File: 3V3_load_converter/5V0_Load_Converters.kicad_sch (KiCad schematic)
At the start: 78 parts, among them J19 N/A, J20 N/A, Q1 SI2302DDS-T1-GE3, Q11 EPC2016C, Q12 EPC2016C, Q2 SI2302DDS-T1-GE3, Q3 EPC2016C, Q4 EPC2016C, U22 INA199C3DCKR, U23 LTC3833EUDC#TRPBF, U26 LTC3833EUDC#TRPBF

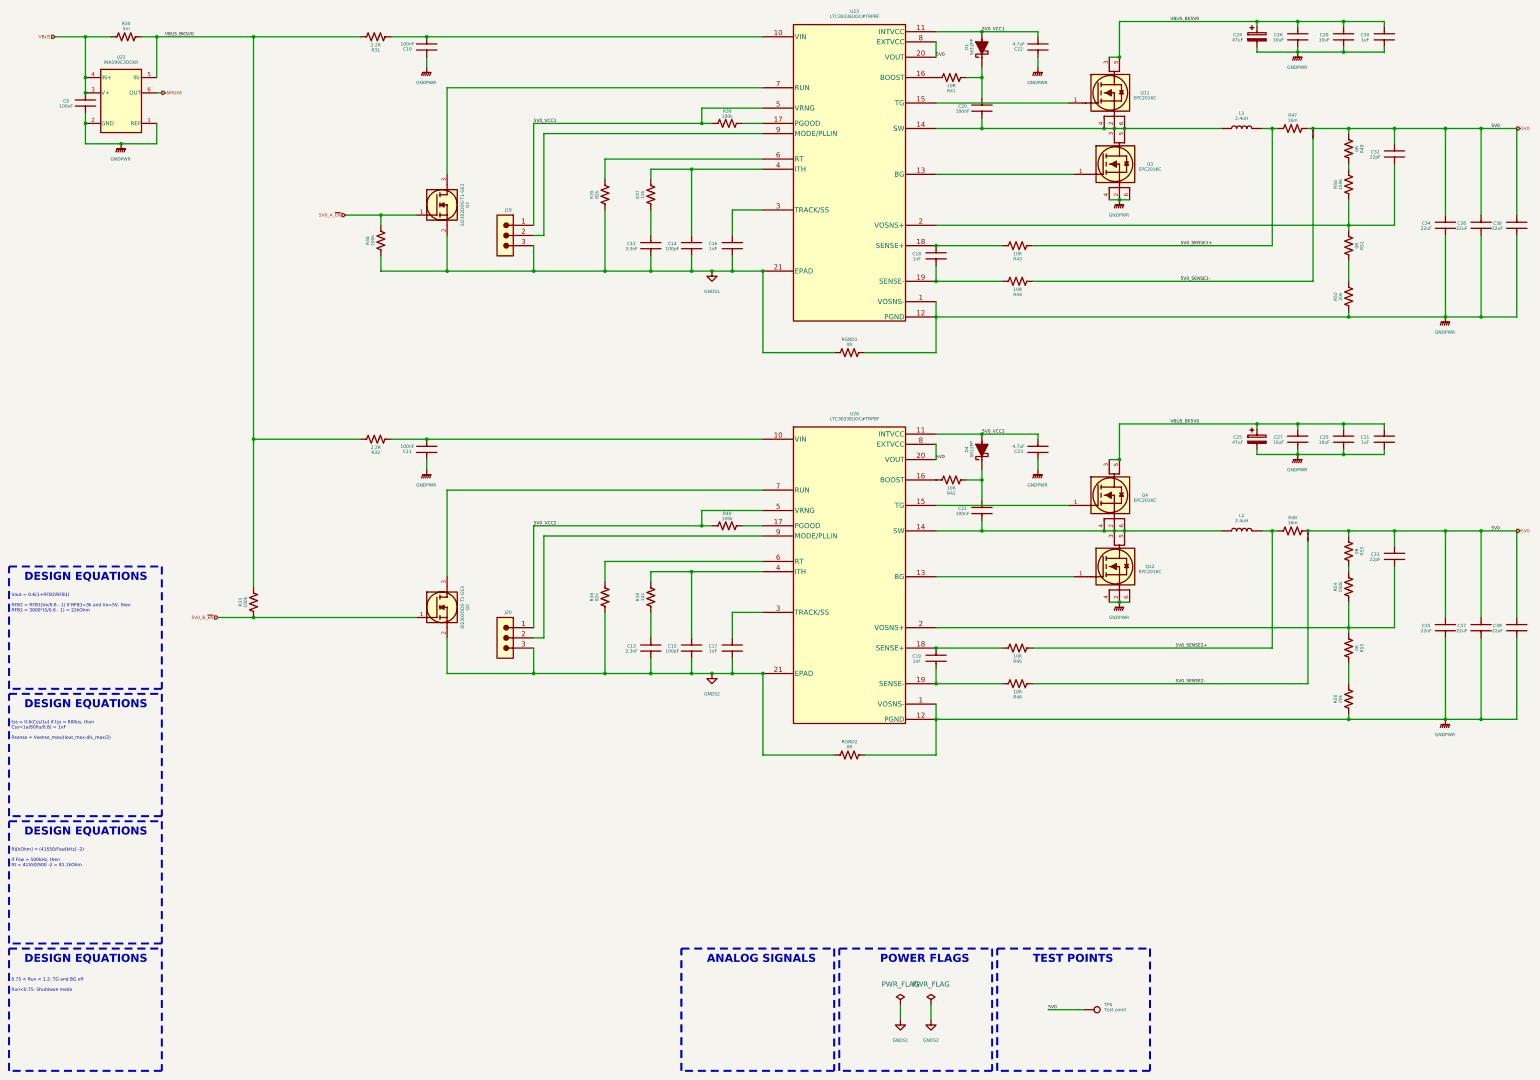
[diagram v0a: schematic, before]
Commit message: update
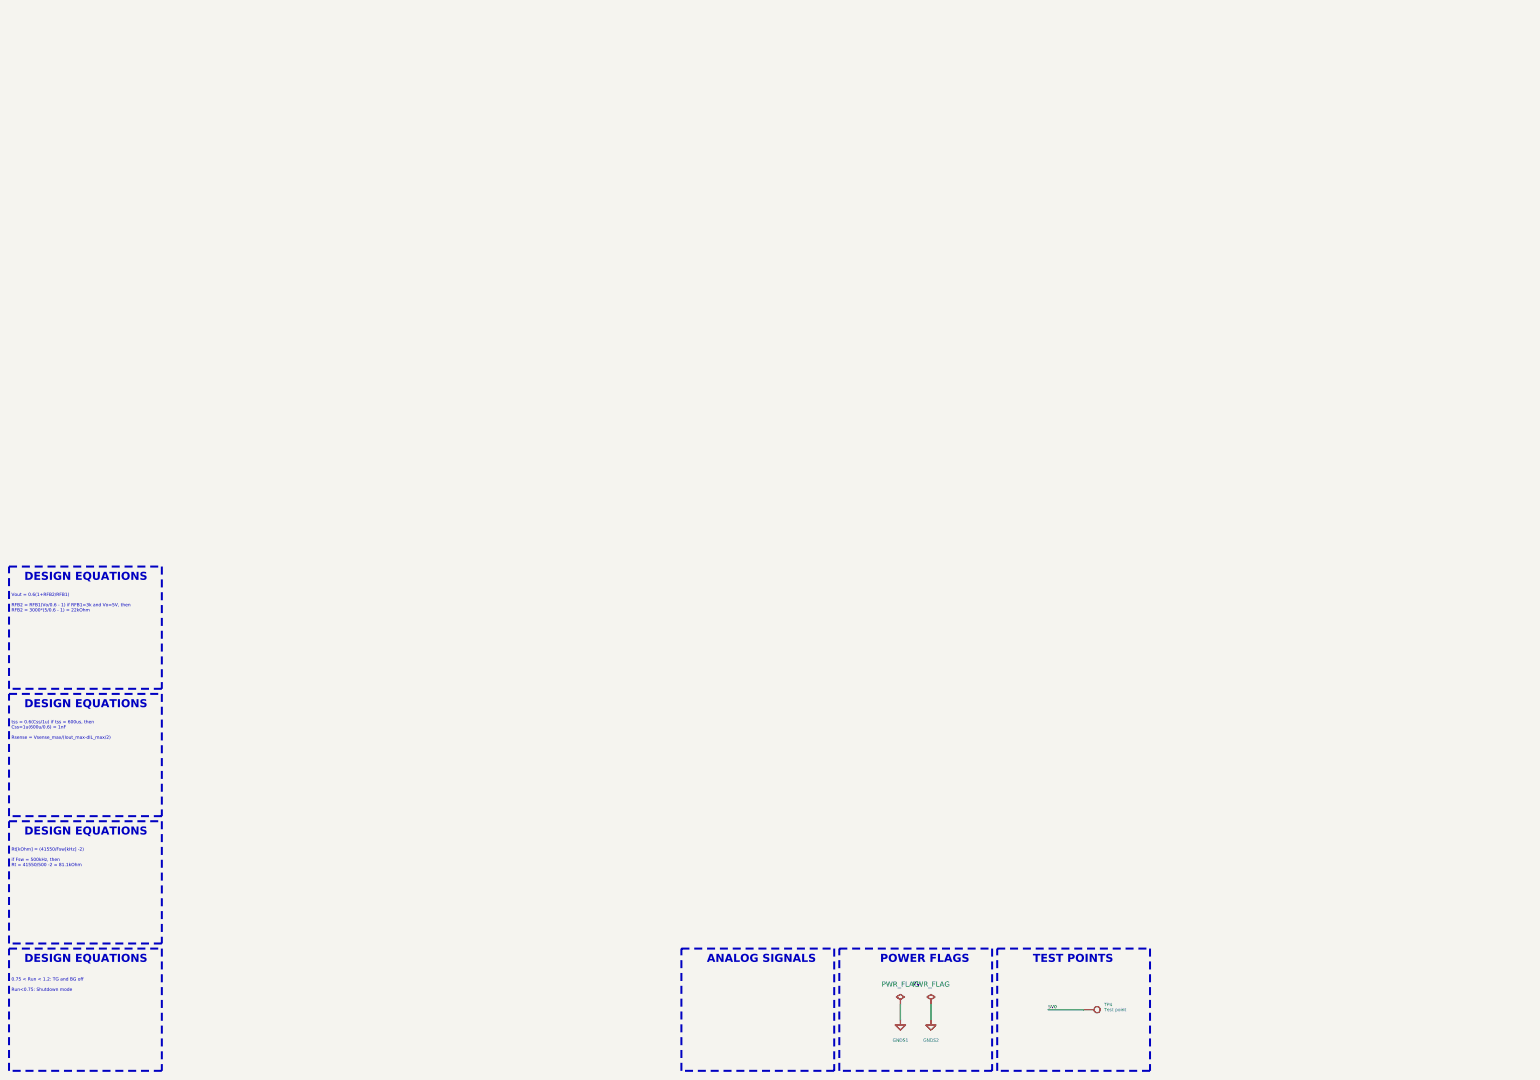
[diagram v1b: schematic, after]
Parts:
- removed C10, C11, C20, C21, C9: 100nF, footprints:CAP0603, symbol C0603C104K5RACTU:C0603C104K5RACTU
- removed C12, C13: 3.3nF, footprints:CAP0603, symbol C0603C332J5GACAUTO:C0603C332J5GACAUTO
- removed C14, C15: 100pF, footprints:CAP0603, symbol C0603C101J5GACAUTO:C0603C101J5GACAUTO
- removed C16, C17, C18, C19: 1nF, footprints:CAP0603, symbol C0603C102F3GACTU:C0603C102F3GACTU
- removed C22, C23: 4.7uF, footprints:CAP1210, symbol GCM32ER71H475KA55L:GCM32ER71H475KA55L
- removed C24, C25: 47uF, footprints:CAP2917POL, symbol T495X476K035ATE300:T495X476K035ATE300
- removed C26, C27, C28, C29: 10uF, footprints:CAP1210, symbol C1210C106K5RACTU:C1210C106K5RACTU
- removed C30, C31: 1uF, footprints:CAP0805, symbol C0805C105K5RACTU:C0805C105K5RACTU
- removed C32, C33: 22pF, footprints:CAP0603, symbol C0603C220K5RACAUTO:C0603C220K5RACAUTO
- removed C34, C35, C36, C37, C38, C39: 22uF, footprints:CAP1210, symbol GCM32ER71C226KE19L:GCM32ER71C226KE19L
- removed D1, D4: SS12FP, footprints:SS12FP, symbol SS12FP:SS12FP
- removed J19, J20: N/A, footprints:three_position_jumper, symbol JUMPER_SMD:JUMPER_SMD
- removed JP1, JP2: N/A, footprints:Jumper, symbol JUMPER:JUMPER
- removed L1, L2: 2.4uH, footprints:744325240, symbol 744325240:744325240
- removed Q1, Q2: SI2302DDS-T1-GE3, footprints:SI2302DDS-T1-GE3, symbol SI2302DDS-T1-GE3:SI2302DDS-T1-GE3
- removed Q11, Q12, Q3, Q4: EPC2016C, footprints:EPC2016C, symbol EPC2016C:EPC2016C
- removed R30: 5m, footprints:RES2010, symbol WSL20105L000FEA:WSL20105L000FEA
- removed R31, R32: 2.2R, footprints:RES0603, symbol CRCW06032R20FKEAHP:CRCW06032R20FKEAHP
- removed R33, R34, R39, R40: 100k, footprints:RES0603, symbol CRCW0603100KFKEAHP:CRCW0603100KFKEAHP
- removed R35, R36: 82k, footprints:RES0603, symbol CRCW060382K0FKEA:CRCW060382K0FKEA
- removed R37, R38: 12k, footprints:RES0603, symbol CRCW060312K0FKEAHP:CRCW060312K0FKEAHP
- removed R41, R42, R43, R44, R45, R46: 10R, footprints:RES0603, symbol CRCW060310R0FKEAHP:CRCW060310R0FKEAHP
- removed R47, R48: 16m, footprints:RES2010, symbol WSL2010R0160FEA:WSL2010R0160FEA
- removed R49, R51, R53, R55, RGND1, RGND2: 0R, footprints:RES0603, symbol CRCW06030000Z0EAHP:CRCW06030000Z0EAHP
- removed R50, R54: 150k, footprints:RES0603, symbol CRCW0603150KFKEAHP:CRCW0603150KFKEAHP
- removed R52, R56: 20k, footprints:RES0603, symbol CRCW060320K0FKEAHP:CRCW060320K0FKEAHP
- removed U22: INA199C3DCKR, footprints:INA199C3DCKR, symbol INA199C3DCKR:INA199C3DCKR
- removed U23, U26: LTC3833EUDC#TRPBF, footprints:LTC3833EUDC#TRPBF, symbol LTC3833EUDC#TRPBF:LTC3833EUDC#TRPBF
